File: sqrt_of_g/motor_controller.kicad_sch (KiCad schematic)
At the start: 25 parts, among them U9 DRV8332DKDR

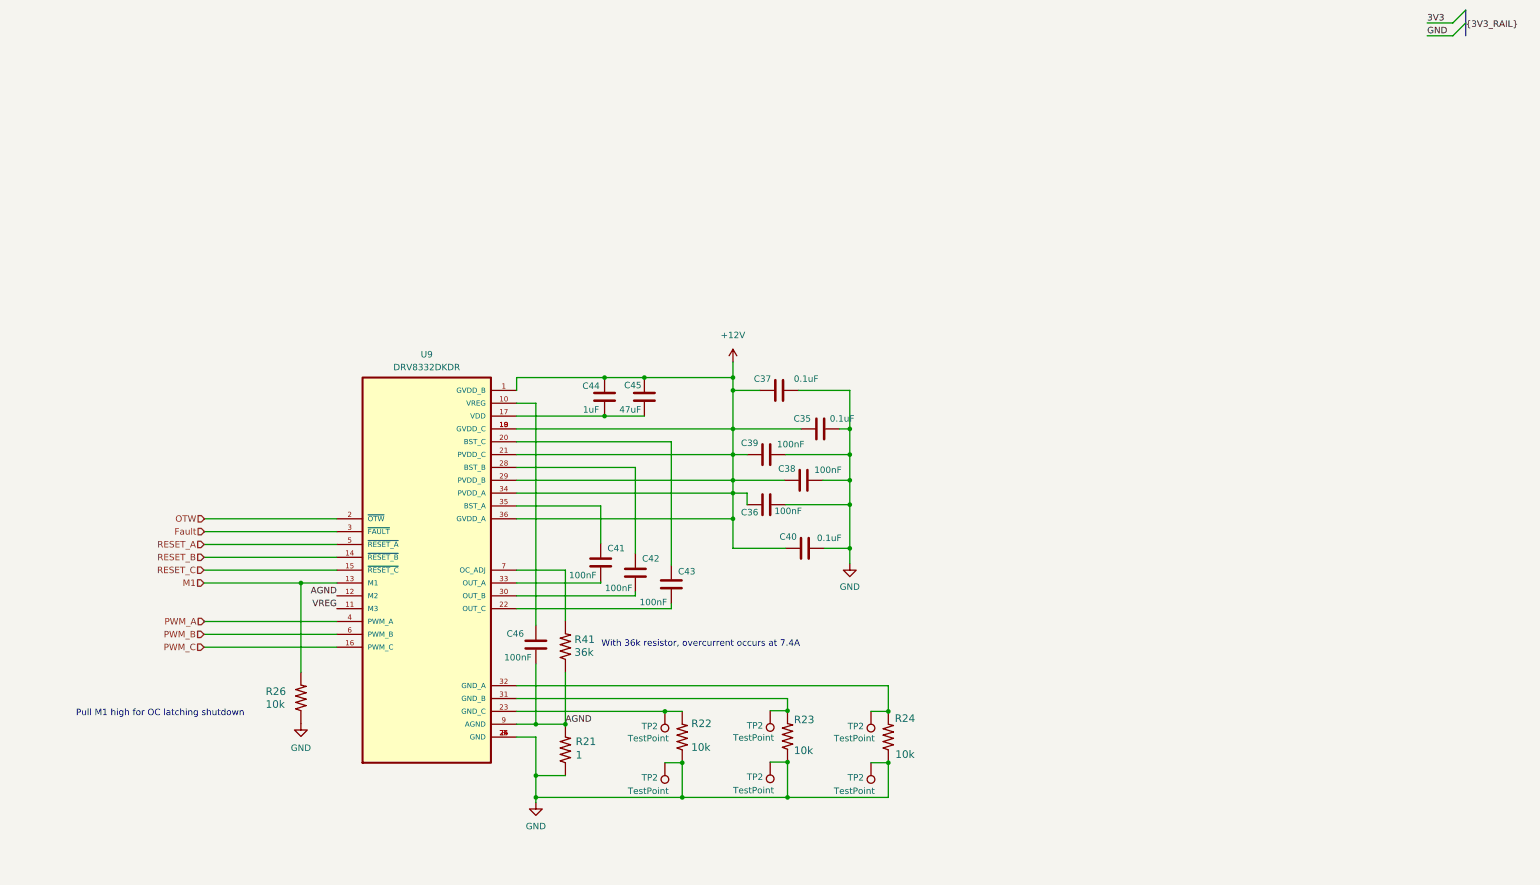
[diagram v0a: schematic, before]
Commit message: update main board
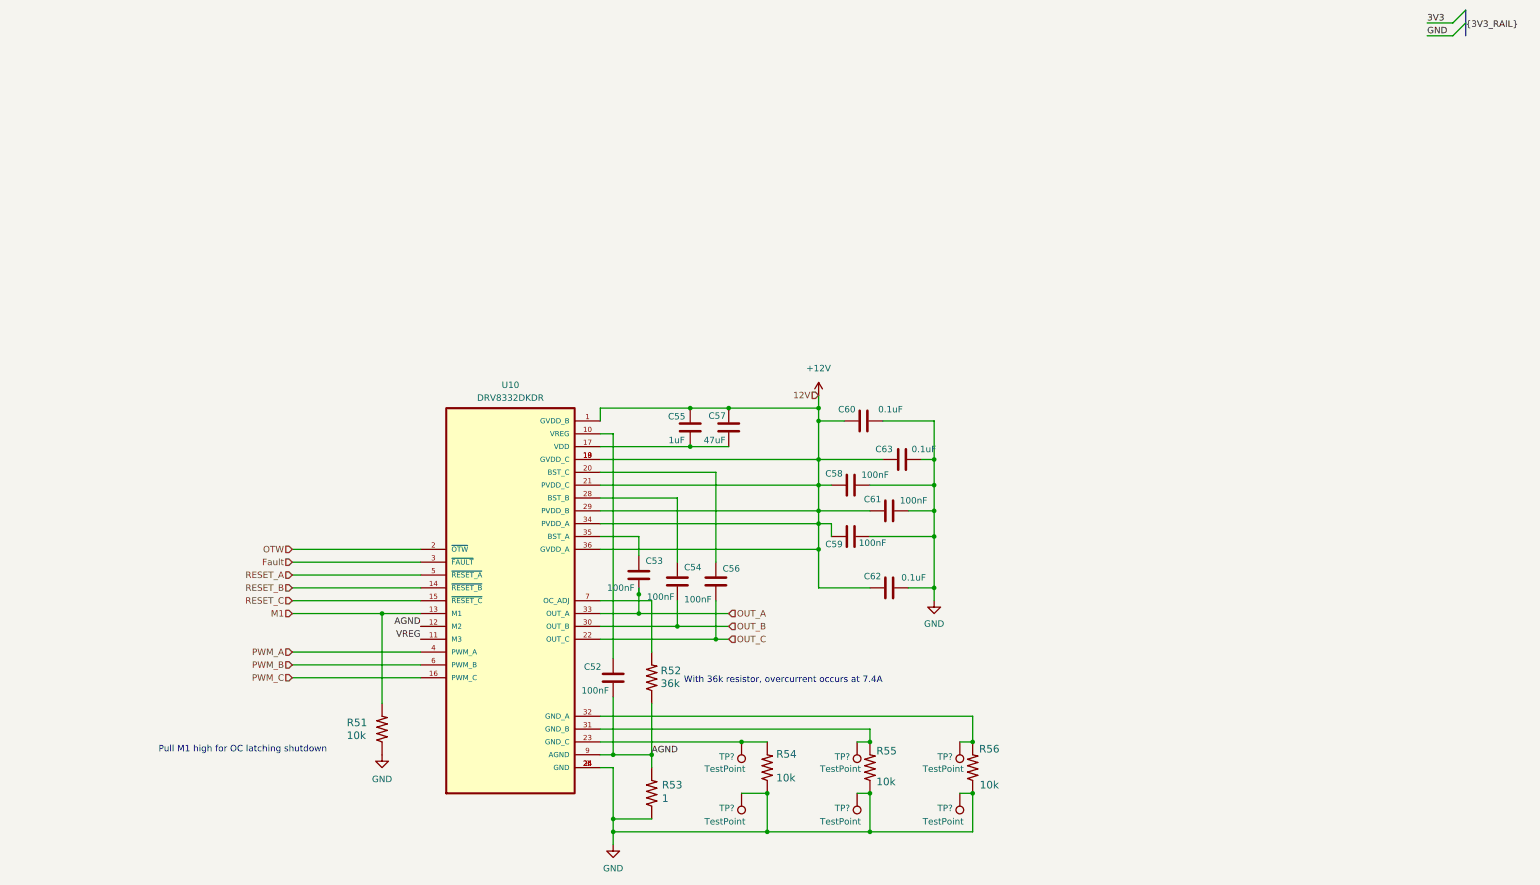
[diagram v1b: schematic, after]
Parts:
- renumbered C46 to C52, C41 to C53, C42 to C54, C44 to C55, C43 to C56, C45 to C57, C39 to C58, C36 to C59, C37 to C60, C38 to C61, C40 to C62, C35 to C63, R26 to R51, R41 to R52, R21 to R53, R22 to R54, R23 to R55, R24 to R56, TP2 to TP?, U9 to U10
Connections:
- net OUT_B: now reaches C54.1, U10.30 (OUT_B)
- net OUT_C: now reaches C56.1, U10.22 (OUT_C)
- net OUT_A: now reaches C53.1, U10.33 (OUT_A)
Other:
- moved on the sheet: C52, C53, C54, C55, C56, C57, C58, C59, C60, C61, C62, C63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
